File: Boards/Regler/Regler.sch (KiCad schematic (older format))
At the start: 21 parts, among them P1 CONN_2, P2 CONN_3, P3 CONN_3, P4 CONN_3, P5 CONN_3, P6 CONN_3, SW1 SP3T

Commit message: Anoden-Stabi auf eigenes Board, Endstufe Layouttest
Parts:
- RL1, RL2, RL3: footprint w_relay:relay_40.52 -> Relays_ThroughHole:Relay_DPDT_Schrack-RT2_RM5mm
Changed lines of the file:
@@
 F 0 "RL1" H 5250 1450 50  0000 L CNN
 F 1 "FINDER-30.22" H 5250 1350 50  0000 L CNN
-F 2 "w_relay:relay_40.52" H 4400 1300 60  0001 C CNN
+F 2 "Relays_ThroughHole:Relay_DPDT_Schrack-RT2_RM5mm" H 4400 1300 60  0001 C CNN
 F 3 "" H 4400 1300 60  0000 C CNN
 	1    4400 1300
@@
 F 0 "RL2" H 5250 3050 50  0000 L CNN
 F 1 "FINDER-30.22" H 5250 2950 50  0000 L CNN
-F 2 "w_relay:relay_40.52" H 4400 2900 60  0001 C CNN
+F 2 "Relays_ThroughHole:Relay_DPDT_Schrack-RT2_RM5mm" H 4400 2900 60  0001 C CNN
 F 3 "" H 4400 2900 60  0000 C CNN
 	1    4400 2900
@@
 F 0 "RL3" H 5250 4650 50  0000 L CNN
 F 1 "FINDER-30.22" H 5250 4550 50  0000 L CNN
-F 2 "w_relay:relay_40.52" H 4400 4500 60  0001 C CNN
+F 2 "Relays_ThroughHole:Relay_DPDT_Schrack-RT2_RM5mm" H 4400 4500 60  0001 C CNN
 F 3 "" H 4400 4500 60  0000 C CNN
 	1    4400 4500

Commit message: New Potis
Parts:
- removed RL1, RL2, RL3: FINDER-30.22, Relays_ThroughHole:Relay_DPDT_Schrack-RT2_RM5mm, symbol FINDER-30.22
- added K1, K2, K3: IM00, w_relay:relay_gq-pth, symbol IM00
- RV1, RV2: footprint Potentiometers:Potentiometer_Alps-RK16-double -> Potentiometer_Alps_RKxxx:Potentiometer_Alps-RK271-double
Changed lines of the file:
@@
-$EndComp
-$Comp
-L FINDER-30.22 RL1
-U 1 1 55DA4CFF
-P 4400 1300
-F 0 "RL1" H 5250 1450 50  0000 L CNN
-F 1 "FINDER-30.22" H 5250 1350 50  0000 L CNN
-F 2 "Relays_ThroughHole:Relay_DPDT_Schrack-RT2_RM5mm" H 4400 1300 60  0001 C CNN
-F 3 "" H 4400 1300 60  0000 C CNN
-	1    4400 1300
-	0    1    1    0
-$EndComp
-$Comp
-L FINDER-30.22 RL2
-U 1 1 55DA4D68
-P 4400 2900
-F 0 "RL2" H 5250 3050 50  0000 L CNN
-F 1 "FINDER-30.22" H 5250 2950 50  0000 L CNN
-F 2 "Relays_ThroughHole:Relay_DPDT_Schrack-RT2_RM5mm" H 4400 2900 60  0001 C CNN
-F 3 "" H 4400 2900 60  0000 C CNN
-	1    4400 2900
-	0    1    1    0
-$EndComp
-$Comp
-L FINDER-30.22 RL3
-U 1 1 55DA4DBF
-P 4400 4500
-F 0 "RL3" H 5250 4650 50  0000 L CNN
-F 1 "FINDER-30.22" H 5250 4550 50  0000 L CNN
-F 2 "Relays_ThroughHole:Relay_DPDT_Schrack-RT2_RM5mm" H 4400 4500 60  0001 C CNN
-F 3 "" H 4400 4500 60  0000 C CNN
-	1    4400 4500
-	0    1    1    0
 $EndComp
 $Comp
@@
 F 0 "RV2" H 7060 4310 50  0000 C CNN
 F 1 "Alps 20k log" H 7190 3700 50  0000 C CNN
-F 2 "Potentiometers:Potentiometer_Alps-RK16-double" H 6900 4000 60  0001 C CNN
+F 2 "Potentiometer_Alps_RKxxx:Potentiometer_Alps-RK271-double" H 6900 4000 60  0001 C CNN
 F 3 "" H 6900 4000 60  0000 C CNN
 	1    6900 4000
@@
 F 0 "RV1" H 6360 4310 50  0000 C CNN
 F 1 "Alps 50k lin" H 6490 3700 50  0000 C CNN
-F 2 "Potentiometers:Potentiometer_Alps-RK16-double" H 6200 4000 60  0001 C CNN
+F 2 "Potentiometer_Alps_RKxxx:Potentiometer_Alps-RK271-double" H 6200 4000 60  0001 C CNN
 F 3 "" H 6200 4000 60  0000 C CNN
 	1    6200 4000
@@
 Wire Wire Line
 	4700 4000 4700 4300
+$Comp
+L IM00 K2
+U 1 1 57F85FBB
+P 4400 2900
+F 0 "K2" H 5250 3050 50  0000 L CNN
+F 1 "IM00" H 5250 2950 50  0000 L CNN
+F 2 "w_relay:relay_gq-pth" H 4400 2900 50  0001 C CNN
+F 3 "" H 4400 2900 50  0000 C CNN
+	1    4400 2900
+	0    1    1    0
+$EndComp
+$Comp
+L IM00 K1
+U 1 1 57F861A3
+P 4400 1300
+F 0 "K1" H 5250 1450 50  0000 L CNN
+F 1 "IM00" H 5250 1350 50  0000 L CNN
+F 2 "w_relay:relay_gq-pth" H 4400 1300 50  0001 C CNN
+F 3 "" H 4400 1300 50  0000 C CNN
+	1    4400 1300
+	0    1    1    0
+$EndComp
+$Comp
+L IM00 K3
+U 1 1 57F8622B
+P 4400 4500
+F 0 "K3" H 5250 4650 50  0000 L CNN
+F 1 "IM00" H 5250 4550 50  0000 L CNN
+F 2 "w_relay:relay_gq-pth" H 4400 4500 50  0001 C CNN
+F 3 "" H 4400 4500 50  0000 C CNN
+	1    4400 4500
+	0    1    1    0
+$EndComp
 $EndSCHEMATC

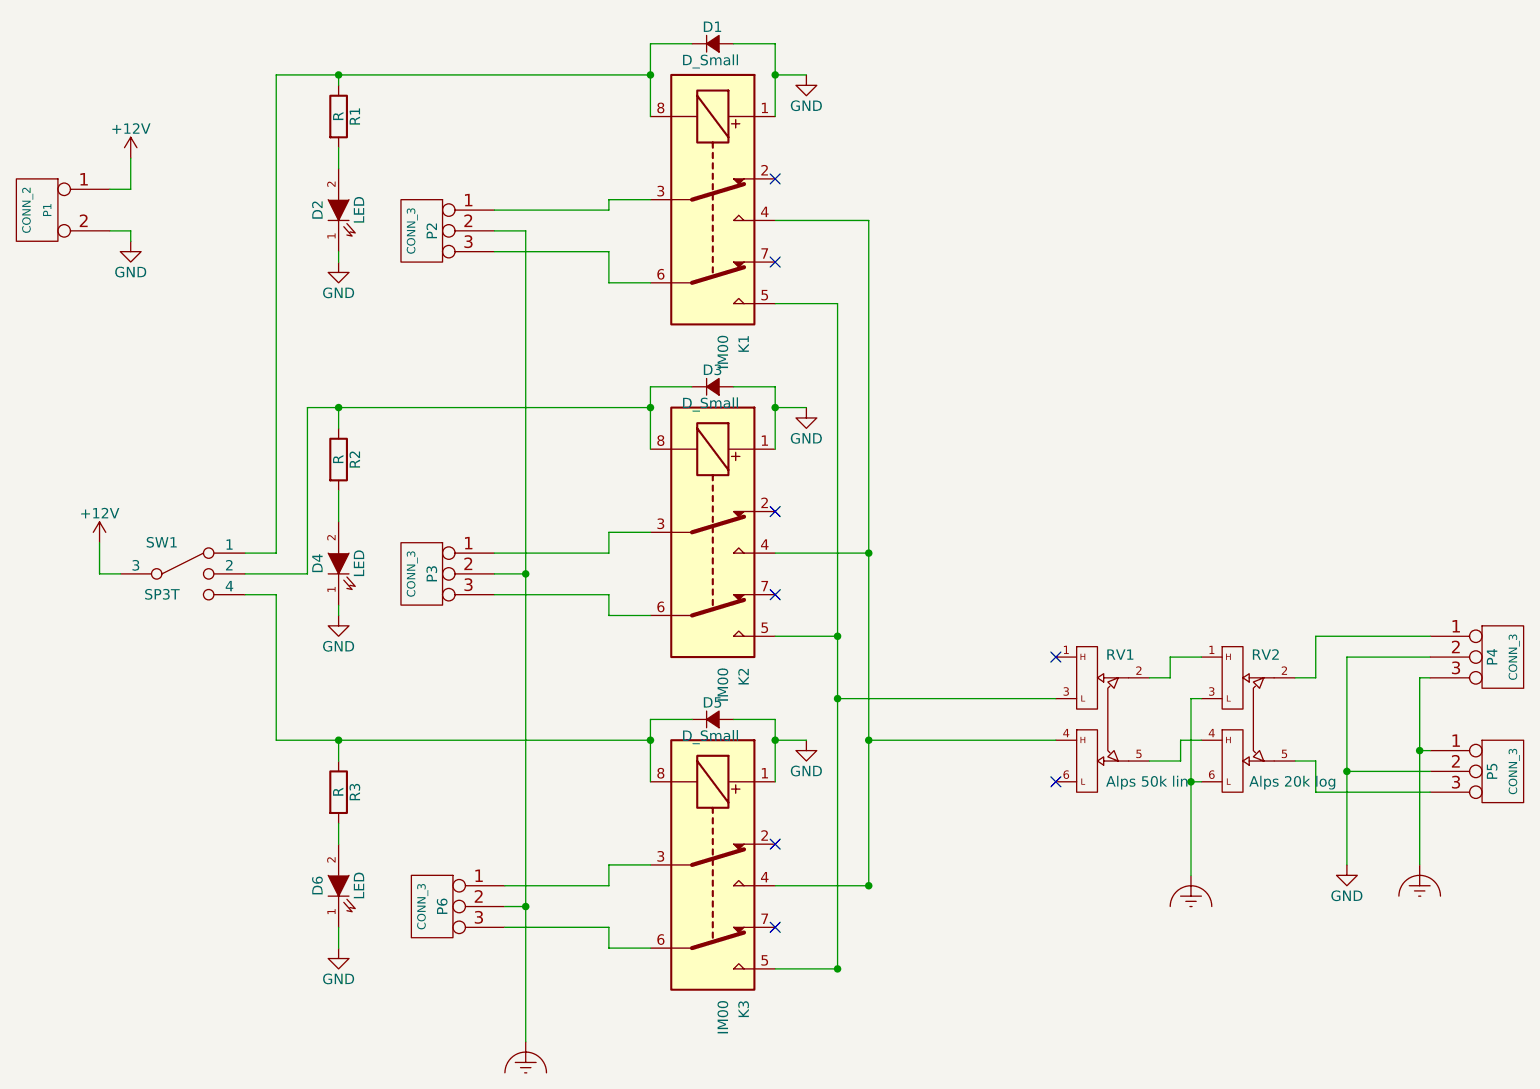
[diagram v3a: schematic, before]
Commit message: Work in Progress
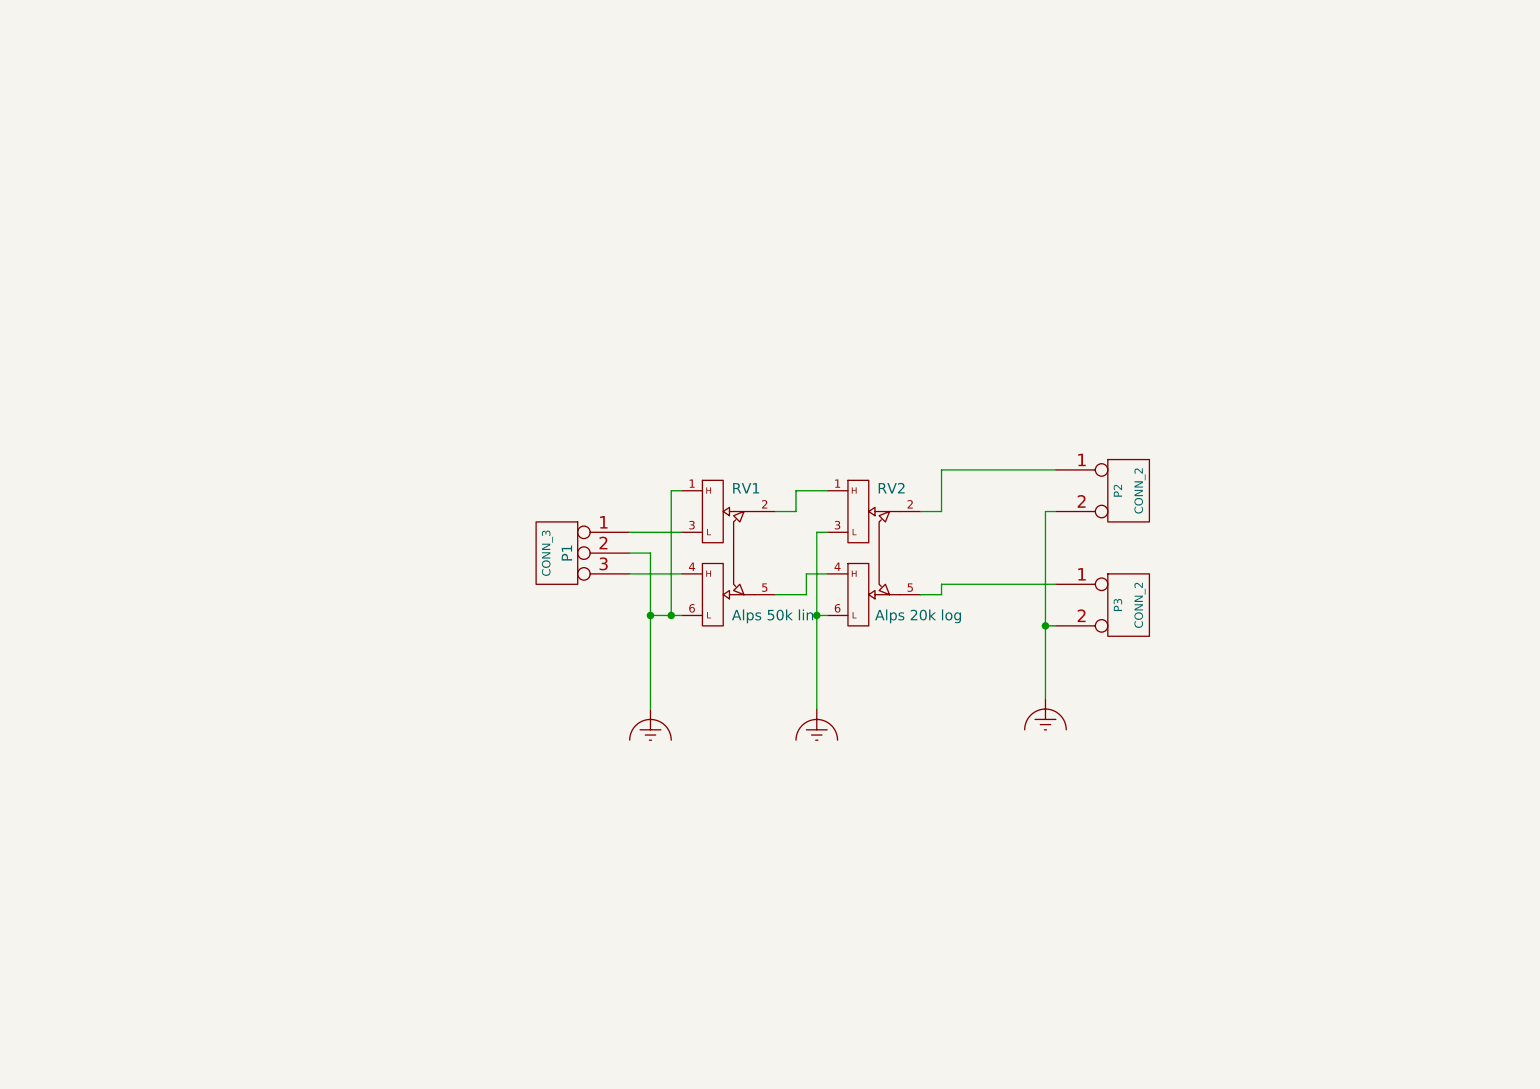
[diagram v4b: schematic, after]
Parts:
- removed D1, D3, D5: D_Small, w_pth_diodes:diode_do15, symbol D_Small
- removed D2, D4, D6: LED, LEDs:LED-3MM, symbol LED
- removed K1, K2, K3: IM00, w_relay:relay_gq-pth, symbol IM00
- removed P1: CONN_2, MiniUniversalMate-N-LokSockets_13Aug2012:MiniUniversalMate-N-LokSocket_2PinHorizontal_13Aug2012, symbol CONN_2
- removed P2, P3, P4, P5, P6: CONN_3, MiniUniversalMate-N-LokSockets_13Aug2012:MiniUniversalMate-N-LokSocket_3PinVertical_12Aug2012, symbol CONN_3
- removed R1, R2, R3: R, Resistors_ThroughHole:Resistor_Horizontal_RM10mm, symbol R
- removed SW1: SP3T, w_switch:pcb_push_xiejia_pb-11d14, symbol SP3T
- added P1: CONN_3, Sockets_Mini-Universal:MiniUniversalMate-N-LokSocket_3PinVertical, symbol CONN_3
- added P2, P3: CONN_2, Sockets_Mini-Universal:MiniUniversalMate-N-LokSocket_2PinVertical, symbol CONN_2
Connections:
- net Earth_Clean: now also RV1.1, RV1.6, P1.2 (P2), P2.2 (P2), P3.2 (P2)
- net at RV2.2: now also P2.1 (P1)
- net at RV2.5: now also P3.1 (P1)
- net at RV1.3: now also P1.1 (P1)
- net at RV1.4: now also P1.3 (P3)
- no-connect marks 8 -> 0
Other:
- moved on the sheet: RV1, RV2

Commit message: Work in Progress
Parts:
- P1: footprint Sockets_Mini-Universal:MiniUniversalMate-N-LokSocket_3PinVertical -> Connectors_Molex:Molex_KK-6410-03_03x2.54mm_Straight; symbol CONN_3 -> borniers:CONN_3
- P2, P3: footprint Sockets_Mini-Universal:MiniUniversalMate-N-LokSocket_2PinVertical -> Connectors_Molex:Molex_KK-6410-02_02x2.54mm_Straight; symbol CONN_2 -> borniers:CONN_2
- RV1, RV2: symbol DUAL_POT -> Regler-rescue:DUAL_POT
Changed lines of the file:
@@
-EESchema Schematic File Version 2
-LIBS:power
-LIBS:device
-LIBS:transistors
-LIBS:conn
-LIBS:linear
-LIBS:regul
-LIBS:74xx
-LIBS:cmos4000
-LIBS:adc-dac
-LIBS:memory
-LIBS:xilinx
-LIBS:microcontrollers
-LIBS:dsp
-LIBS:microchip
-LIBS:analog_switches
-LIBS:motorola
-LIBS:texas
-LIBS:intel
-LIBS:audio
-LIBS:interface
-LIBS:digital-audio
-LIBS:philips
-LIBS:display
-LIBS:cypress
-LIBS:siliconi
-LIBS:opto
-LIBS:atmel
-LIBS:contrib
-LIBS:valves
-LIBS:borniers
-LIBS:relays
-LIBS:GR_relays
-LIBS:reed_relais
+EESchema Schematic File Version 4
 LIBS:Regler-cache
-EELAYER 25 0
+EELAYER 26 0
 EELAYER END
 $Descr A4 11693 8268
@@
 $EndDescr
 $Comp
-L DUAL_POT RV2
+L Regler-rescue:DUAL_POT RV2
 U 1 1 55DA80EE
 P 5100 3200
@@
 $EndComp
 $Comp
-L DUAL_POT RV1
+L Regler-rescue:DUAL_POT RV1
 U 1 1 55DA8395
 P 4400 3200
@@
 $EndComp
 $Comp
-L Earth_Clean #PWR01
+L power:Earth_Clean #PWR01
 U 1 1 55DAD2B4
 P 4900 3950
@@
 $EndComp
 $Comp
-L Earth_Clean #PWR02
+L power:Earth_Clean #PWR02
 U 1 1 55DAD3CD
 P 6000 3900
@@
 	4950 3100 4900 3100
 Wire Wire Line
-	4900 3100 4900 3950
+	4900 3100 4900 3500
 Wire Wire Line
 	4950 3500 4900 3500
@@
 	5500 3350 5500 3400
 Wire Wire Line
-	6000 3000 6000 3900
+	6000 3000 6000 3550
 $Comp
-L CONN_3 P1
+L borniers:CONN_3 P1
 U 1 1 581F54BF
 P 3650 3200
 F 0 "P1" V 3600 3200 50  0000 C CNN
 F 1 "CONN_3" V 3700 3200 40  0000 C CNN
-F 2 "Sockets_Mini-Universal:MiniUniversalMate-N-LokSocket_3PinVertical" H 3650 3200 60  0001 C CNN
+F 2 "Connectors_Molex:Molex_KK-6410-03_03x2.54mm_Straight" H 3650 3200 60  0001 C CNN
 F 3 "" H 3650 3200 60  0000 C CNN
 	1    3650 3200
@@
 	4000 3300 4250 3300
 $Comp
-L Earth_Clean #PWR03
+L power:Earth_Clean #PWR03
 U 1 1 581F55B2
 P 4100 3950
@@
 	4000 3200 4100 3200
 Wire Wire Line
-	4100 3200 4100 3950
+	4100 3200 4100 3500
 $Comp
-L CONN_2 P2
+L borniers:CONN_2 P2
 U 1 1 5945B6EB
 P 6400 2900
 F 0 "P2" V 6350 2900 40  0000 C CNN
 F 1 "CONN_2" V 6450 2900 40  0000 C CNN
-F 2 "Sockets_Mini-Universal:MiniUniversalMate-N-LokSocket_2PinVertical" H 6400 2900 60  0001 C CNN
+F 2 "Connectors_Molex:Molex_KK-6410-02_02x2.54mm_Straight" H 6400 2900 60  0001 C CNN
 F 3 "" H 6400 2900 60  0001 C CNN
 	1    6400 2900
@@
 $EndComp
 $Comp
-L CONN_2 P3
+L borniers:CONN_2 P3
 U 1 1 5945B7D4
 P 6400 3450
 F 0 "P3" V 6350 3450 40  0000 C CNN
 F 1 "CONN_2" V 6450 3450 40  0000 C CNN
-F 2 "Sockets_Mini-Universal:MiniUniversalMate-N-LokSocket_2PinVertical" H 6400 3450 60  0001 C CNN
+F 2 "Connectors_Molex:Molex_KK-6410-02_02x2.54mm_Straight" H 6400 3450 60  0001 C CNN
 F 3 "" H 6400 3450 60  0001 C CNN
 	1    6400 3450
@@
 	4200 2900 4200 3500
 Wire Wire Line
-	4100 3500 4250 3500
+	4100 3500 4200 3500
 Connection ~ 4100 3500
 Connection ~ 4200 3500
+Wire Wire Line
+	4900 3500 4900 3950
+Wire Wire Line
+	6000 3550 6000 3900
+Wire Wire Line
+	4100 3500 4100 3950
+Wire Wire Line
+	4200 3500 4250 3500
 $EndSCHEMATC

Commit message: Converted to Kicad 5.1 and Layout changes
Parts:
- P1: symbol borniers:CONN_3 -> Regler-rescue:CONN_3-borniers
- P2, P3: symbol borniers:CONN_2 -> Regler-rescue:CONN_2-borniers
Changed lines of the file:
@@
 	6000 3000 6000 3550
 $Comp
-L borniers:CONN_3 P1
+L Regler-rescue:CONN_3-borniers P1
 U 1 1 581F54BF
 P 3650 3200
@@
 	4100 3200 4100 3500
 $Comp
-L borniers:CONN_2 P2
+L Regler-rescue:CONN_2-borniers P2
 U 1 1 5945B6EB
 P 6400 2900
@@
 $EndComp
 $Comp
-L borniers:CONN_2 P3
+L Regler-rescue:CONN_2-borniers P3
 U 1 1 5945B7D4
 P 6400 3450
